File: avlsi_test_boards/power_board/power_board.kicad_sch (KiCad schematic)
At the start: 4 parts, among them J1 PJ-102AH, J2 PJ-102AH, J3 Conn_02x07_Odd_Even, J4 Conn_02x07_Odd_Even

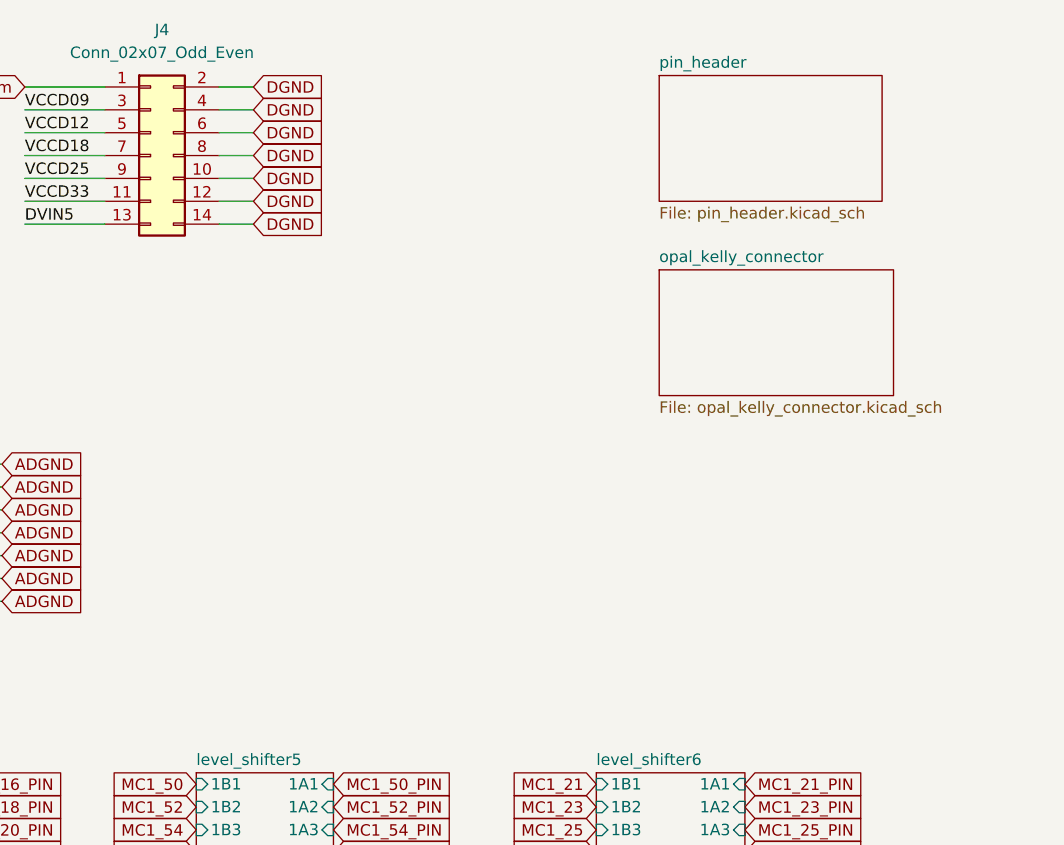
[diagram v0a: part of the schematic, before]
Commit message: Add initial layout stuff
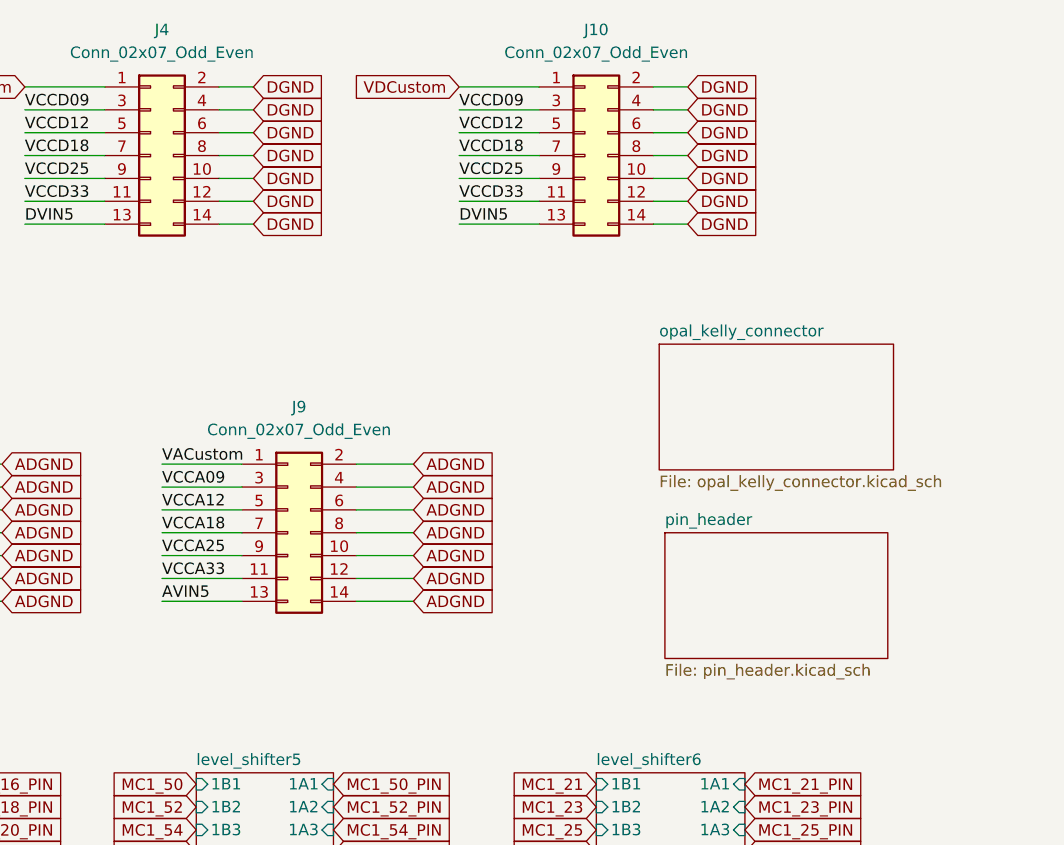
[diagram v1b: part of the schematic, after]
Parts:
- added J10, J9: Conn_02x07_Odd_Even, Connector_PinHeader_2.54mm:PinHeader_2x07_P2.54mm_Vertical, symbol Connector_Generic:Conn_02x07_Odd_Even
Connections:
- net ADGND: now also J9.10 (Pin_10), J9.12 (Pin_12), J9.14 (Pin_14), J9.2 (Pin_2), J9.4 (Pin_4), J9.6 (Pin_6), J9.8 (Pin_8)
- net AVIN5: now also J9.13 (Pin_13)
- net DGND: now also J10.10 (Pin_10), J10.12 (Pin_12), J10.14 (Pin_14), J10.2 (Pin_2), J10.4 (Pin_4), J10.6 (Pin_6), J10.8 (Pin_8)
- net DVIN5: now also J10.13 (Pin_13)
- net VACustom: now also J9.1 (Pin_1)
- net VCCA09: now also J9.3 (Pin_3)
- net VCCA12: now also J9.5 (Pin_5)
- net VCCA18: now also J9.7 (Pin_7)
- net VCCA25: now also J9.9 (Pin_9)
- net VCCA33: now also J9.11 (Pin_11)
- net VCCD09: now also J10.3 (Pin_3)
- net VCCD12: now also J10.5 (Pin_5)
- net VCCD18: now also J10.7 (Pin_7)
- net VCCD25: now also J10.9 (Pin_9)
- net VCCD33: now also J10.11 (Pin_11)
- net VDCustom: now also J10.1 (Pin_1)
